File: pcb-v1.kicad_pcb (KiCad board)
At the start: 2 copper layers, 28 parts, among them J1 Conn_01x03_Socket, J10 Screw_Terminal_01x04, J11 Screw_Terminal_01x04, J12 Screw_Terminal_01x04, J13 Screw_Terminal_01x04, J14 Screw_Terminal_01x06, J15 Conn_01x06_Pin, J2 Conn_01x03_Socket, J3 Conn_01x03_Socket, J4 Conn_01x03_Socket, J5 Conn_01x03_Socket, J6 Conn_01x03_Socket, J7 Conn_01x08_Socket, J8 Conn_01x04_Socket, J9 Conn_01x06_Pin

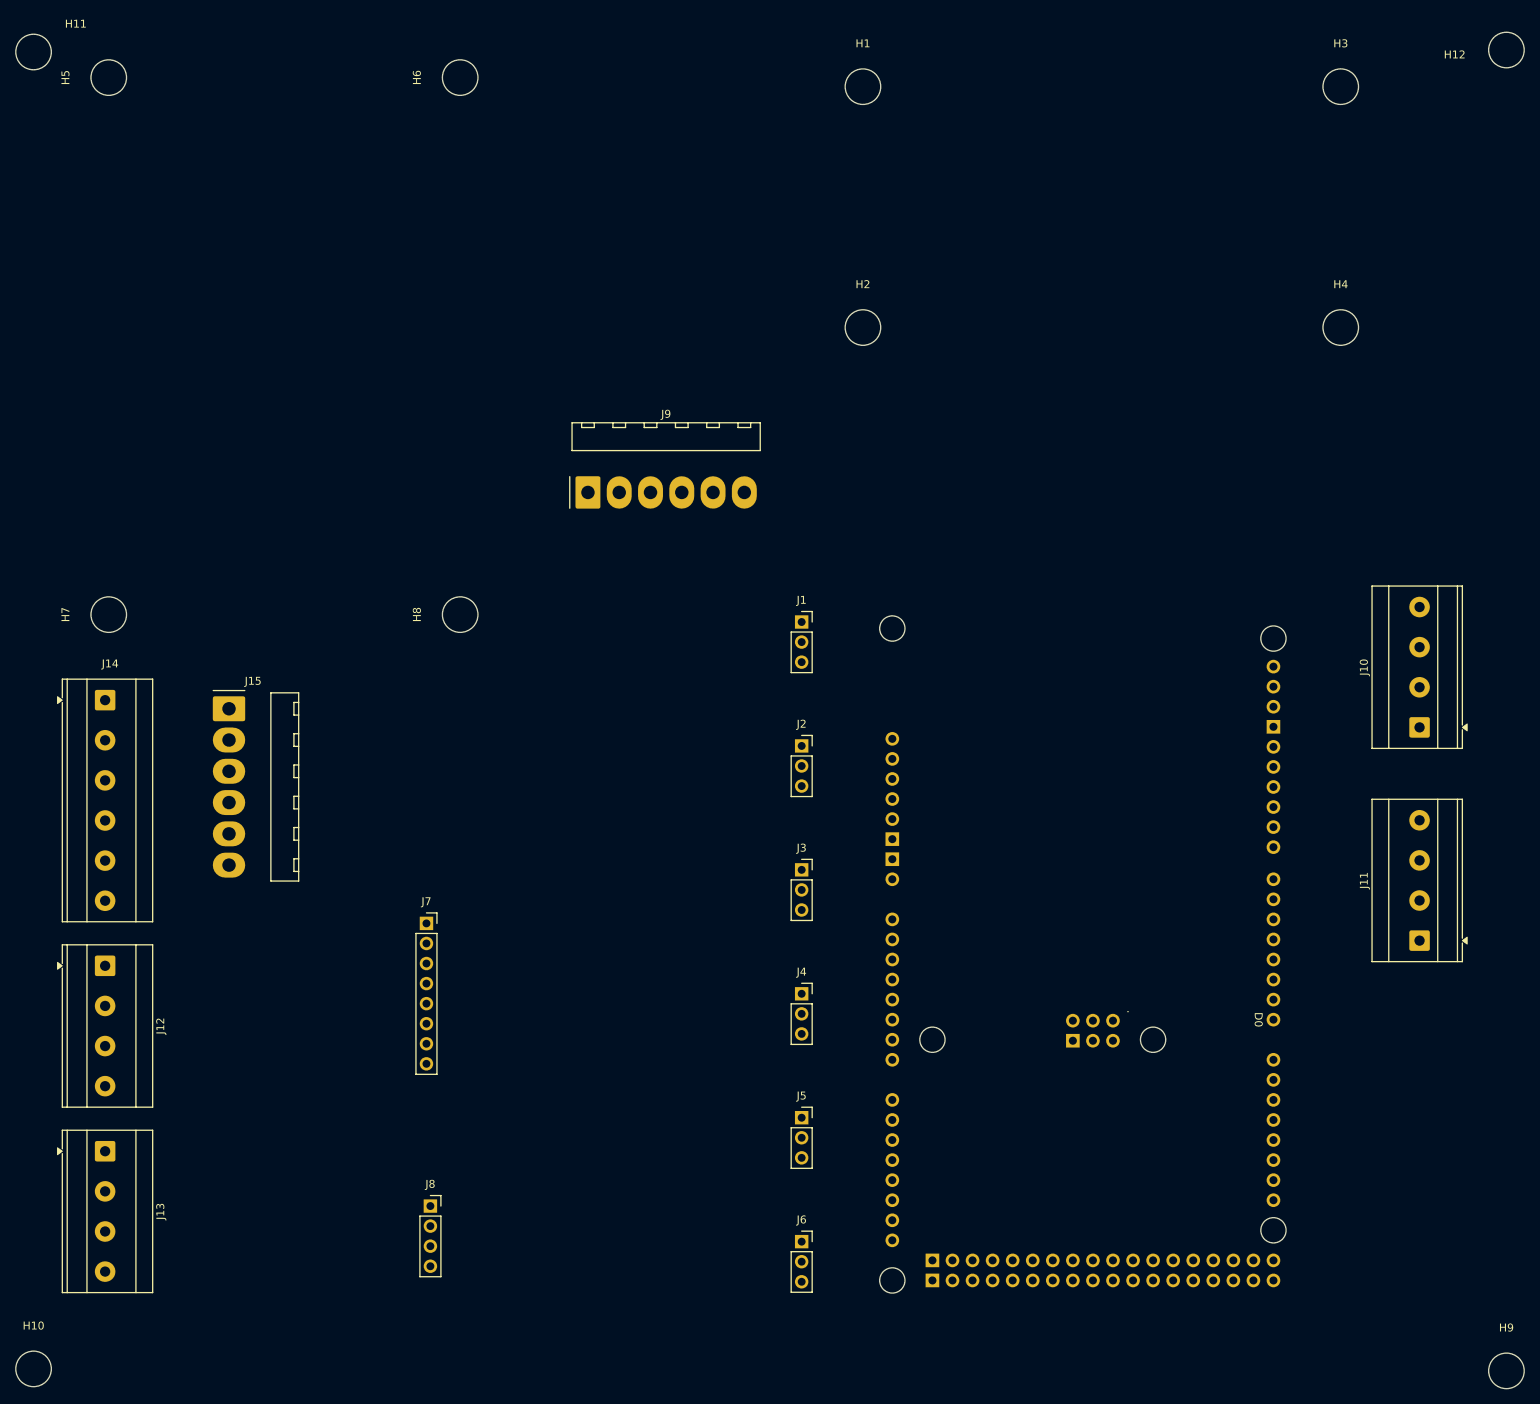
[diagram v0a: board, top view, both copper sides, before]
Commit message: add part finish
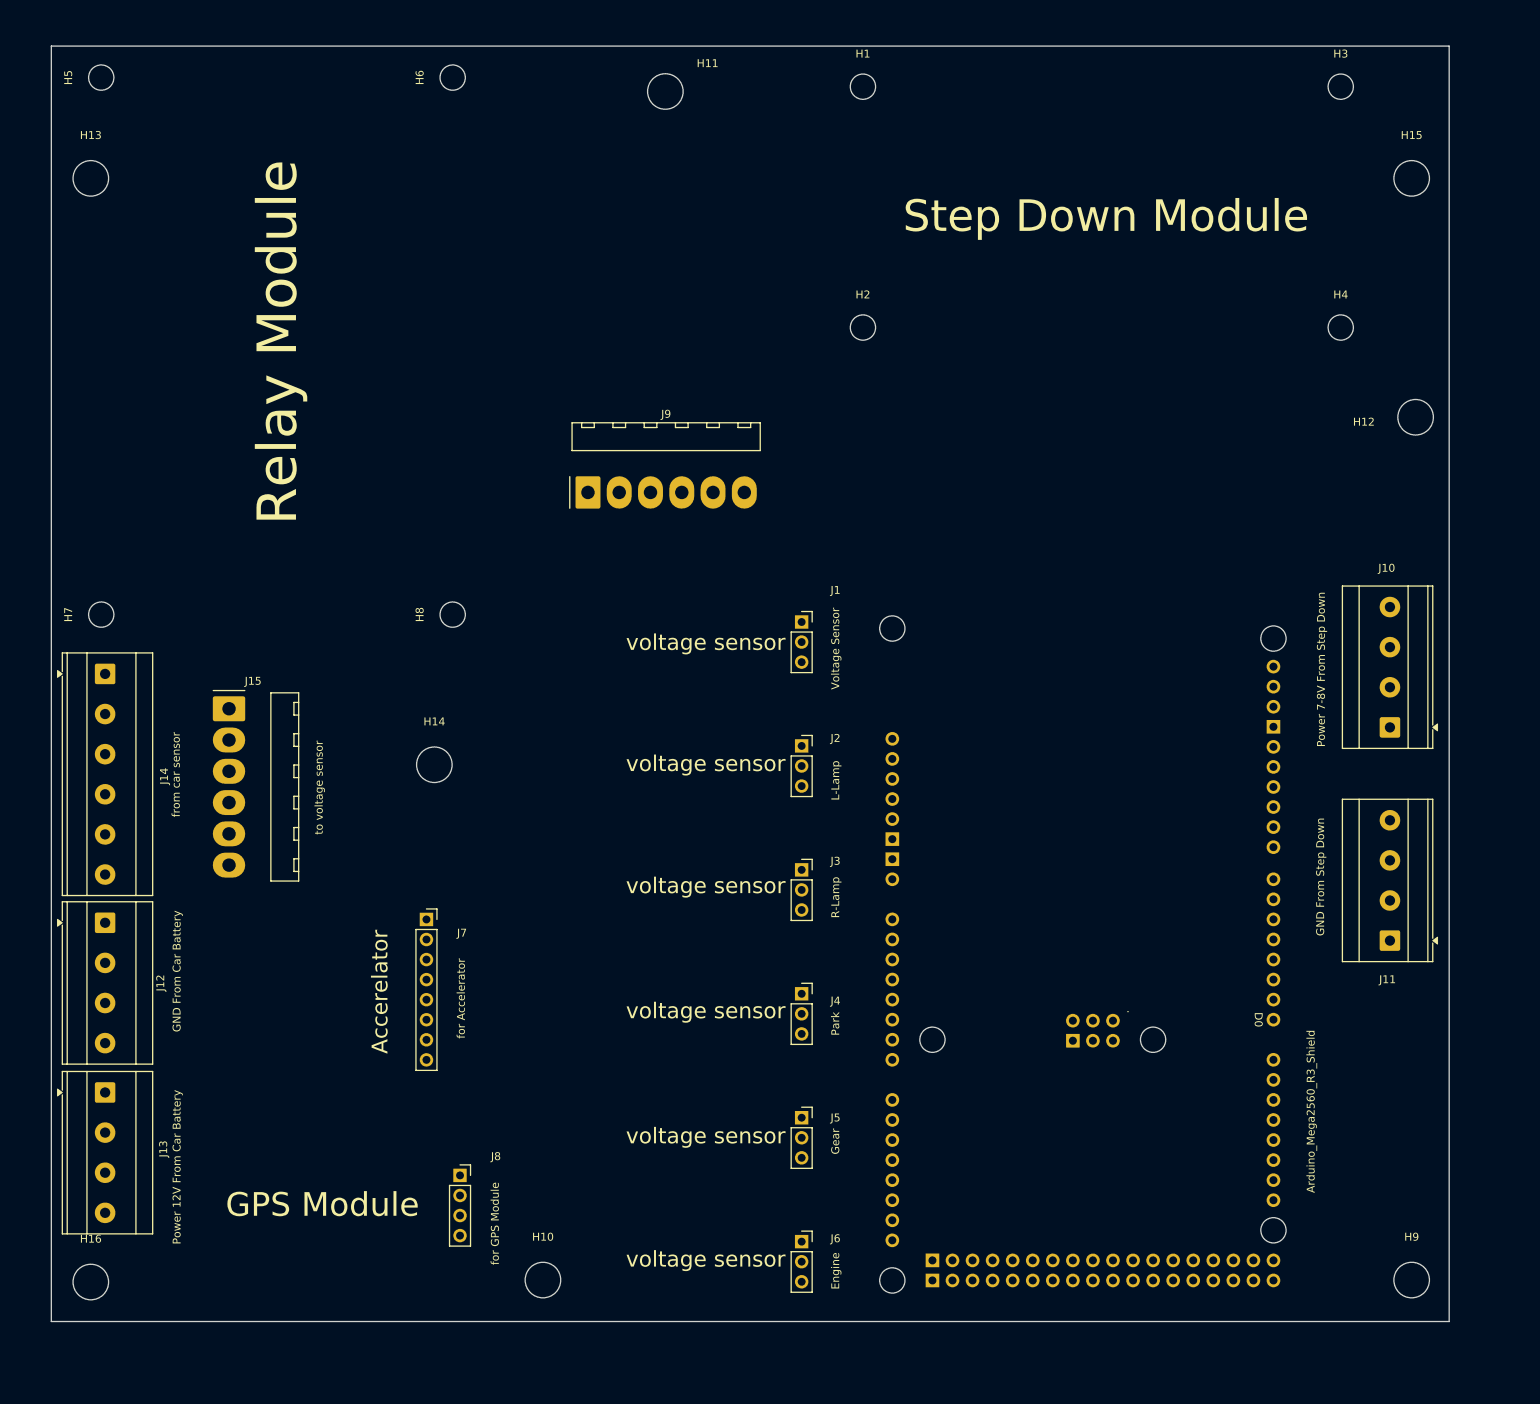
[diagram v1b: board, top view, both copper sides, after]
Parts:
- added H13: MountingHole, MountingHole:MountingHole_4.5mm, F.Cu at (67.5, 33.2)
- added H14: MountingHole, MountingHole:MountingHole_4.5mm, F.Cu at (111.0, 107.5)
- added H15: MountingHole, MountingHole:MountingHole_4.5mm, F.Cu at (234.8, 33.2)
- added H16: MountingHole, MountingHole:MountingHole_4.5mm, F.Cu at (67.5, 173.0)
- H1, H2, H3, H4, H5, H6, H7, H8: footprint MountingHole:MountingHole_4.5mm -> MountingHole:MountingHole_3.2mm_M3
- moved H11 80.2 mm to (140.2, 22.2)
- moved H10 65.5 mm to (124.8, 172.8)
- moved H12 47.9 mm to (235.2, 63.5)
- moved H9 16.6 mm to (234.8, 172.8)
- moved J13 7.44 mm to (69.3, 149.0)
- moved J12 5.45 mm to (69.3, 127.5)
- moved J8 5.40 mm to (114.2, 159.5)
- moved J10 3.75 mm to (232.0, 102.8)
- moved J11 3.75 mm to (232.0, 129.8)
- moved J14 3.32 mm to (69.3, 96.0)
- moved H5 0.95 mm to (68.8, 20.5)
- moved H6 0.95 mm to (113.3, 20.5)
- moved H7 0.95 mm to (68.8, 88.5)
- moved H8 0.95 mm to (113.3, 88.5)
- moved J7 0.50 mm to (110.0, 127.1)
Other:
- board outline added: 177 x 161.5 mm
